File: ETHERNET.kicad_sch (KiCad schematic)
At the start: 23 parts, among them J4 RJ45, U8 LAN8720A, X1 50MHz

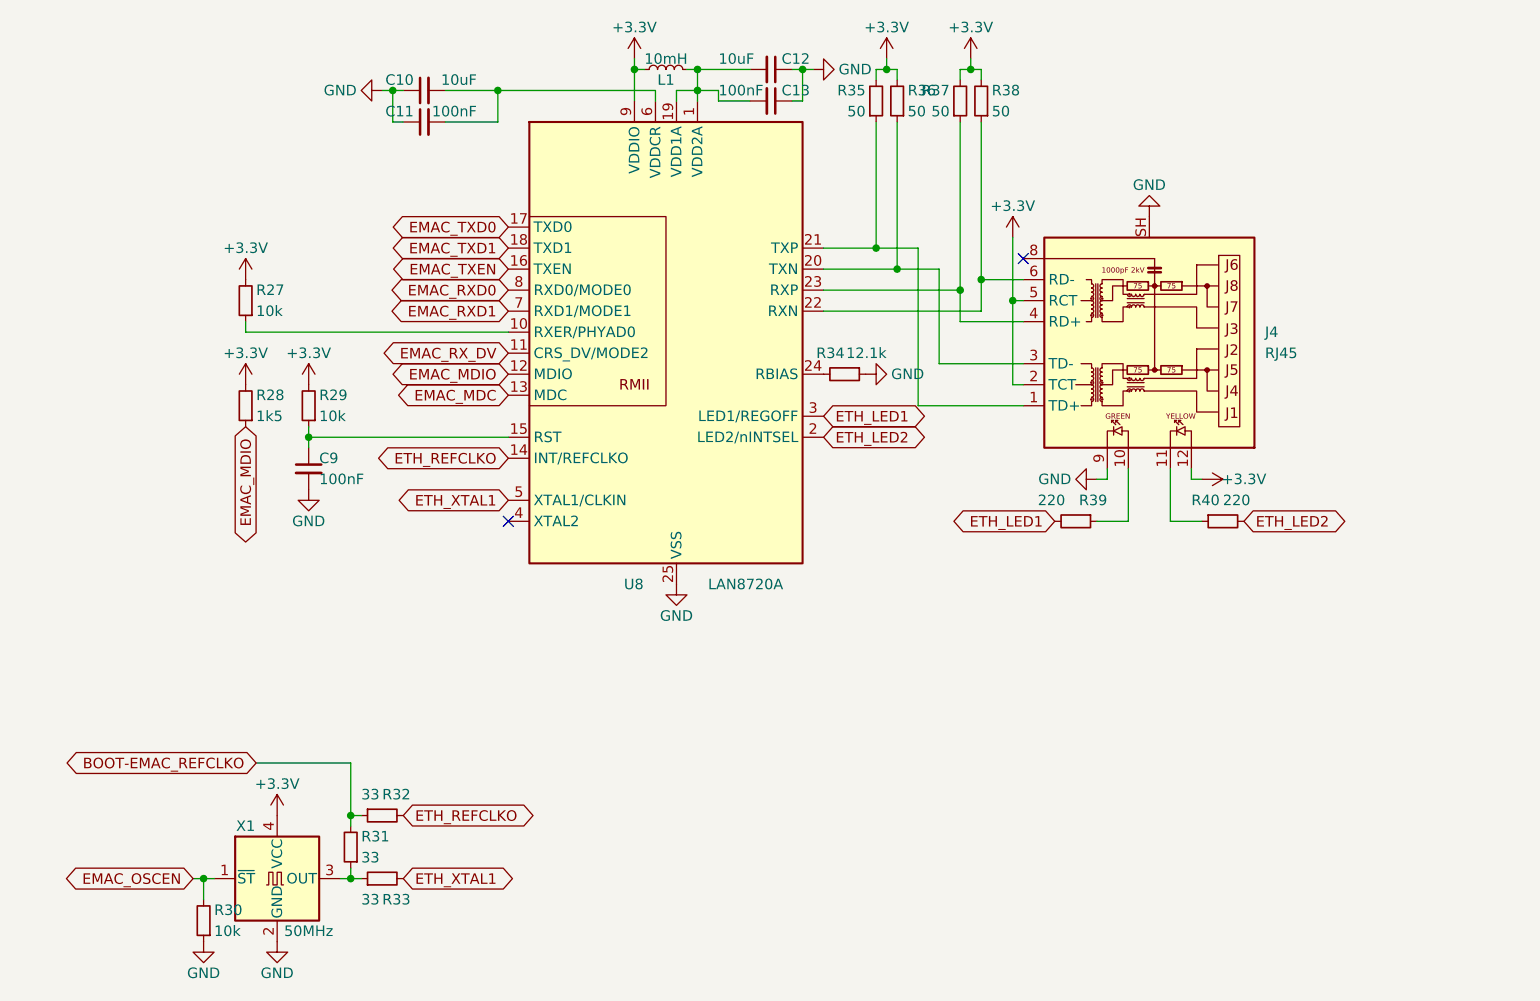
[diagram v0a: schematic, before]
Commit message: Add files via upload
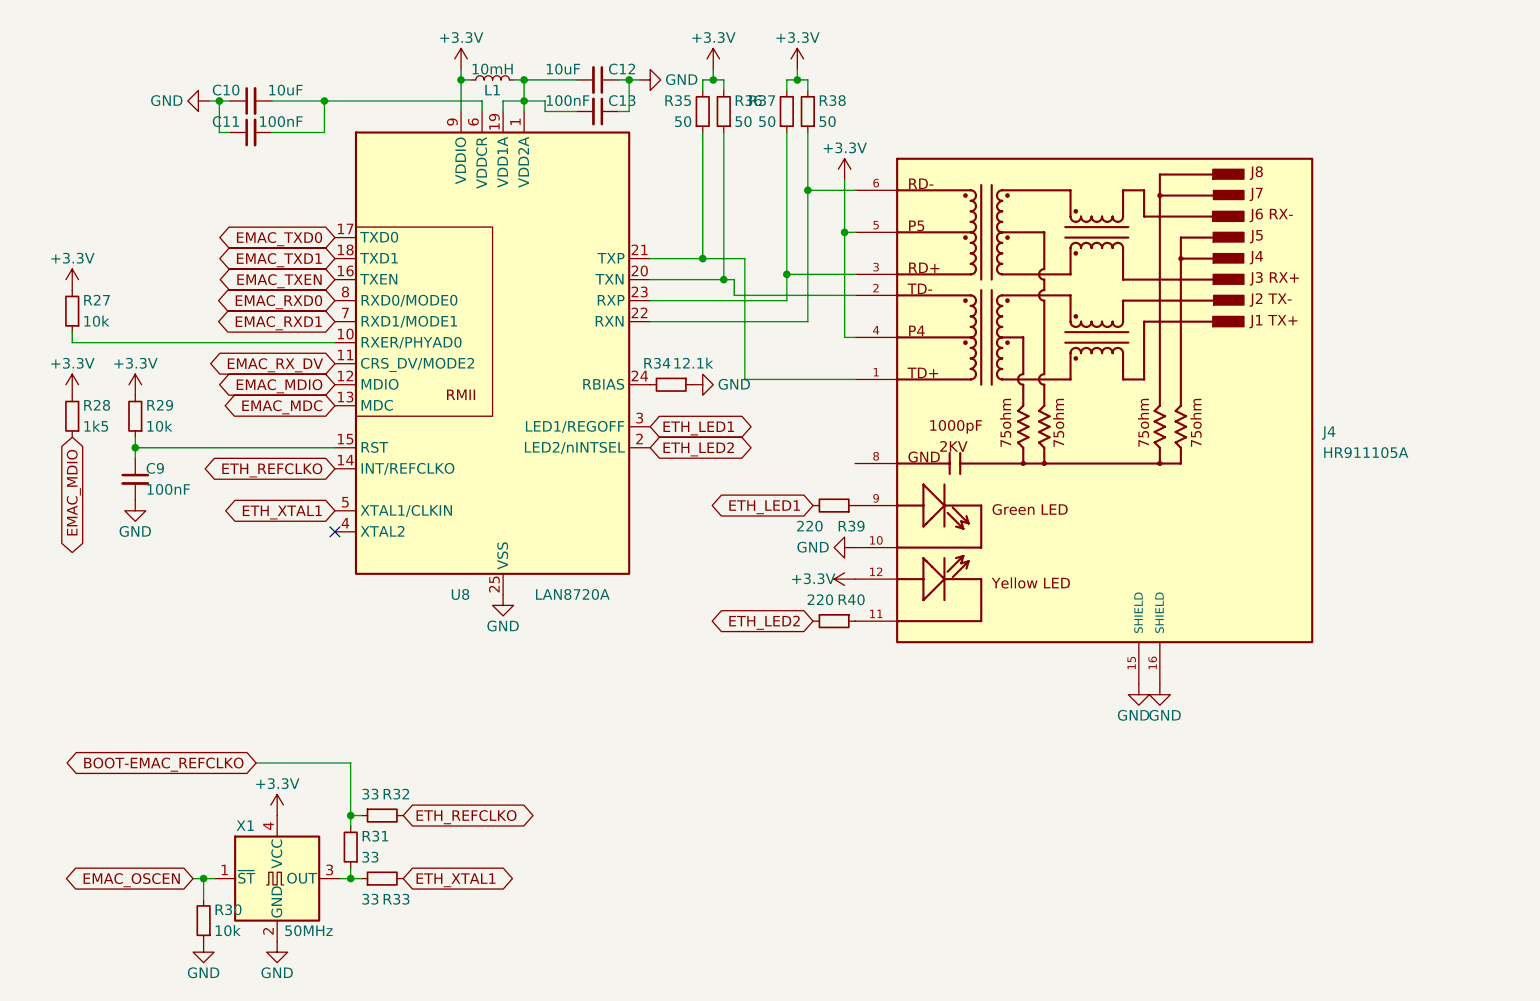
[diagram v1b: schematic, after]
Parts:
- removed J4: RJ45, HANRUN_RJ45LED_HR911105A:HANRUN_RJ45LED_HR911105A, symbol Connector:Wuerth_7499010121A
- added J4: HR911105A, HANRUN_RJ45LED_HR911105A:HANRUN_RJ45LED_HR911105A, symbol HANRUN_RJ45LED_HR911105A:HR911105A
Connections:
- net +3.3V: now also J4.12, J4.4, J4.5
- net GND: now also J4.10, J4.15 (SHIELD), J4.16 (SHIELD)
- net at R38.1, U8.22 (RXN): now also J4.6
- net at R37.1, U8.23 (RXP): now also J4.3
- net at R36.1, U8.20 (TXN): now also J4.2
- net at R35.1, U8.21 (TXP): now also J4.1
- net at R39.1: now also J4.9
- net at R40.1: now also J4.11
- no-connect marks 2 -> 1
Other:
- moved on the sheet: C10, C11, C12, C13, C9, L1, R27, R28, R29, R34, R35, R36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

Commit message: Add files via upload
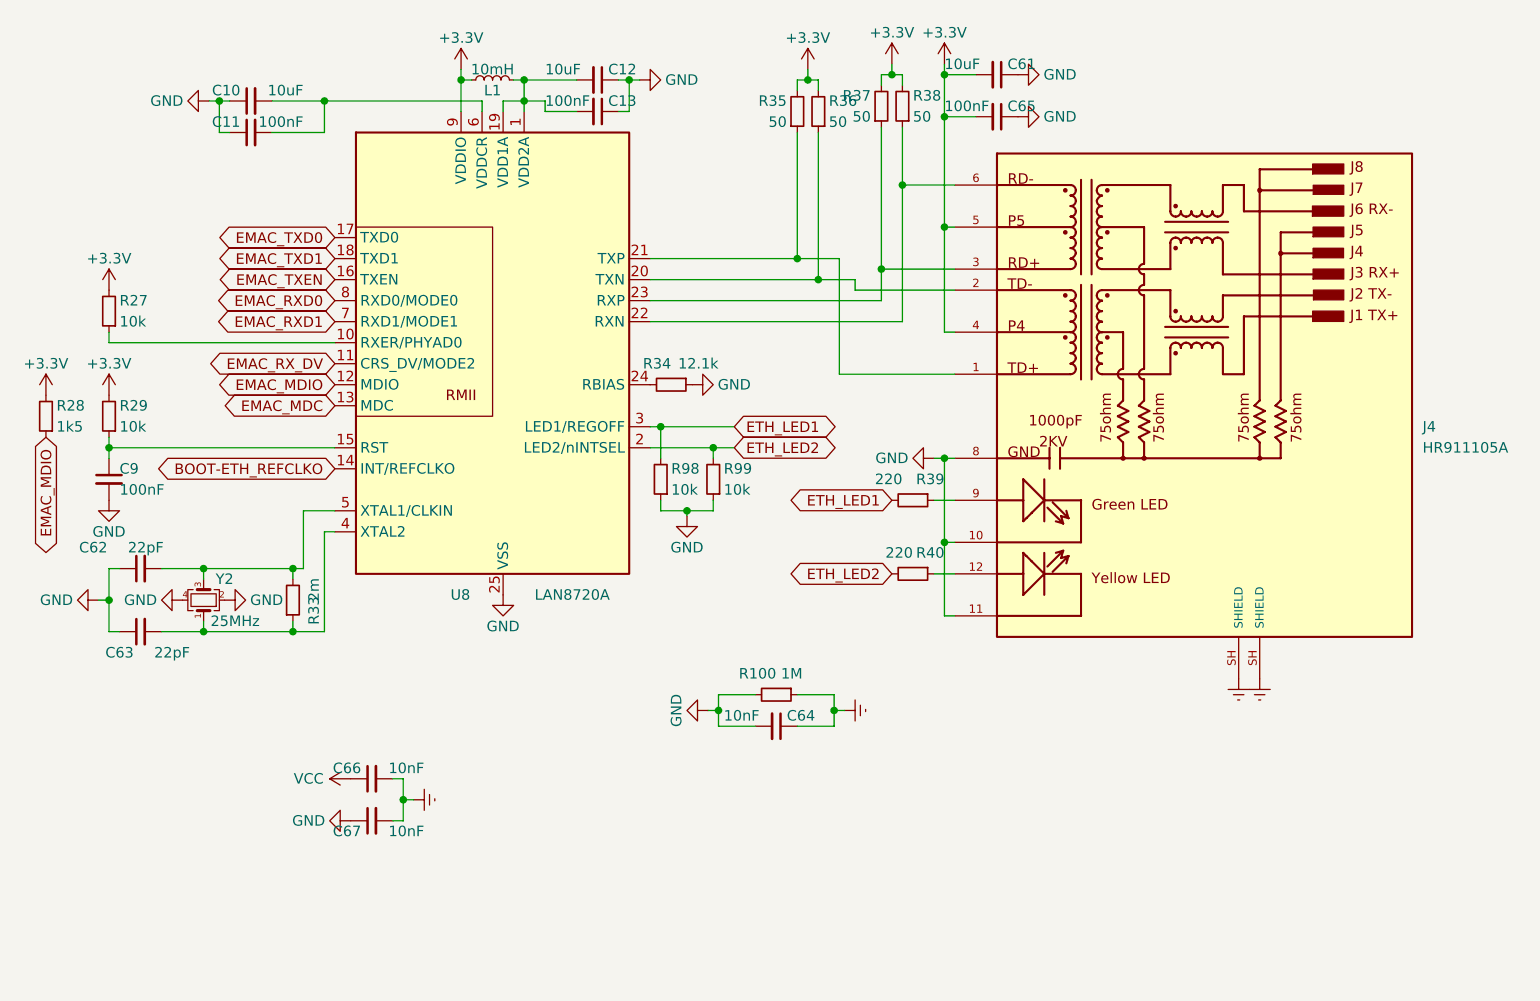
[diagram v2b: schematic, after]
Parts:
- removed R30: 10k, Resistor_SMD:R_0603_1608Metric, symbol Device:R_Small
- removed R31, R32: 33, Resistor_SMD:R_0603_1608Metric, symbol Device:R_Small
- removed X1: 50MHz, Oscillator:Oscillator_SMD_SeikoEpson_SG8002CA-4Pin_7.0x5.0mm, symbol Oscillator:SG-7050CAN
- added C61: 10uF, Capacitor_SMD:C_1206_3216Metric, symbol Device:C_Small
- added C62, C63: 22pF, Capacitor_SMD:C_0603_1608Metric, symbol Device:C_Small
- added C64, C66, C67: 10nF, Capacitor_SMD:C_1206_3216Metric, symbol Device:C_Small
- added C65: 100nF, Capacitor_SMD:C_0603_1608Metric, symbol Device:C_Small
- added R100: 1M, Resistor_SMD:R_1206_3216Metric, symbol Device:R_Small
- added R98, R99: 10k, Resistor_SMD:R_0603_1608Metric, symbol Device:R_Small
- added Y2: 25MHz, Crystal:Crystal_SMD_5032-4Pin_5.0x3.2mm, symbol Device:Crystal_GND24_Small
- R33: value 33 -> 2m
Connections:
- net +3.3V: now also C61.2, C65.2; no longer J4.12
- net ETH_LED1: now also R98.2
- net ETH_LED2: now also R99.2
- net GND: now also J4.11, J4.8, C61.1, C62.1, C63.1, C64.2, C65.1, C67.1, R100.2, R98.1, R99.1, Y2.2, Y2.4; no longer J4.15 (SHIELD), J4.16 (SHIELD)
- net at U8.4 (XTAL2): now also R33.1, C63.2, Y2.1
- net at R40.1: now also J4.12; no longer J4.11
- net ETH_REFCLKO renamed BOOT-ETH_REFCLKO
- net ETH_XTAL1: no longer names the net of R33.2, U8.5 (XTAL1/CLKIN)
- net ETH_XTAL1: now also C62.2, Y2.3
- new net Earth: C64.1, C66.2, C67.2, J4.SH (SHIELD), R100.1
- new net VCC: C66.1
- no-connect marks 1 -> 0
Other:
- moved on the sheet: C9, J4, R27, R28, R29, R35, R36, R37, R38, R39, R40
